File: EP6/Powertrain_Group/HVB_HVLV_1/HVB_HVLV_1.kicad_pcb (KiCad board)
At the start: 2 copper layers, 132 x 62 mm, 20 parts, among them J1 HV+, J2 HV-, J3 from LV, J5 DCDC-, J6 DCDC+, K1 G7L-2A-X DC24, K2 DBT72410, Q1 IXTH6N100D2, U1 PC817

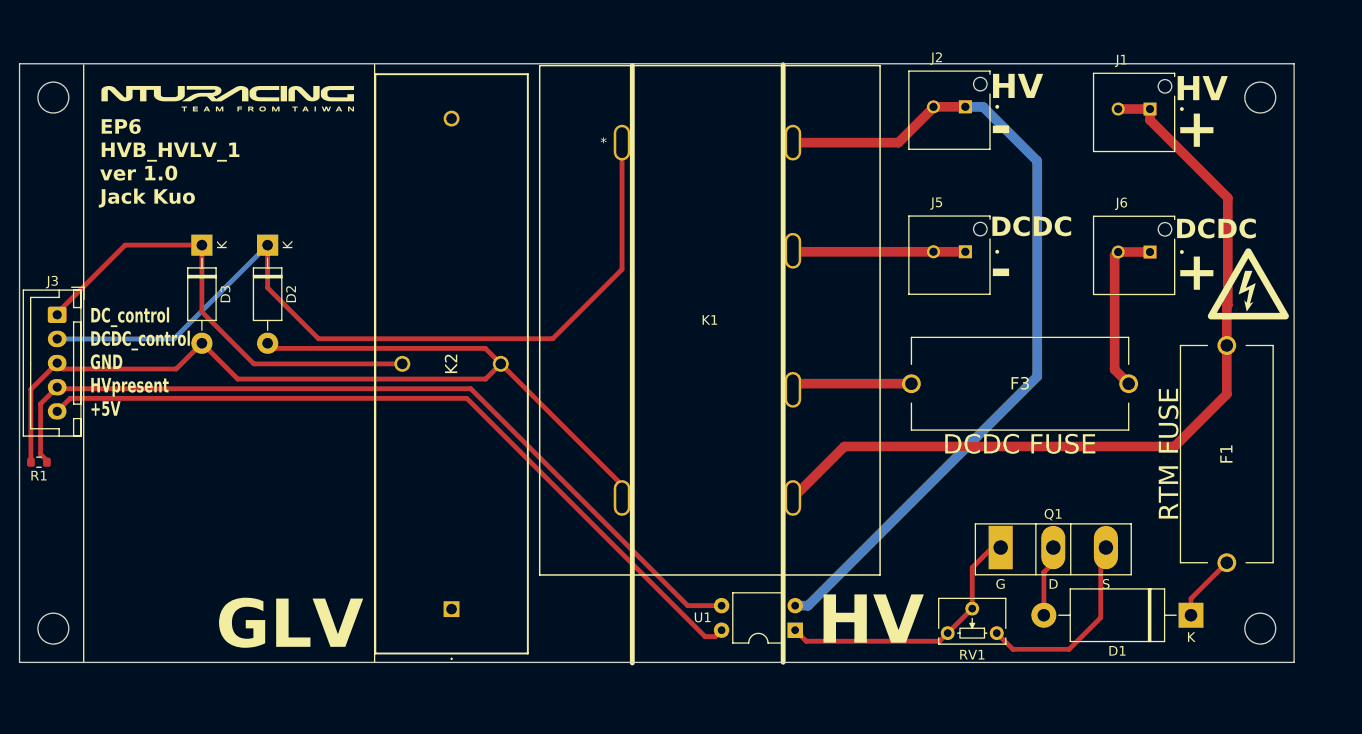
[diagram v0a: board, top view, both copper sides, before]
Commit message: update HVB_HVLV_1 V2.1
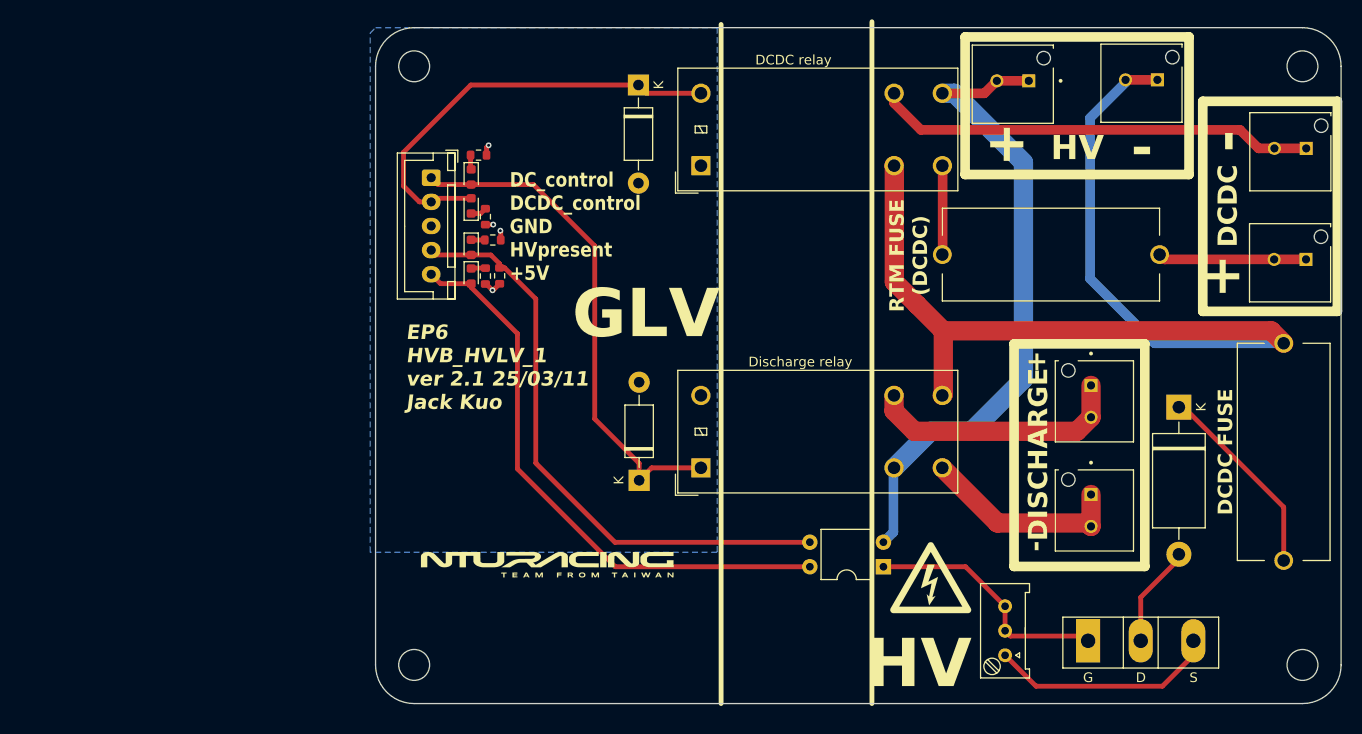
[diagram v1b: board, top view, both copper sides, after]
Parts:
- added D4: RED LED, LED_SMD:LED_0603_1608Metric, F.Cu at (109.9, 47.8)
- added D5: RED LED, LED_SMD:LED_0603_1608Metric, F.Cu at (109.9, 50.7)
- added D6: RED LED, LED_SMD:LED_0603_1608Metric, F.Cu at (109.9, 43.5)
- added D7: RED LED, LED_SMD:LED_0603_1608Metric, F.Cu at (109.9, 40.5)
- added J4: PrechargeRes-, nturt_kicad_lib_EP6:HRS_DF33C-2P-3.3DSA, F.Cu at (174.1, 75.0)
- added J7: PrechargeRes+, nturt_kicad_lib_EP6:HRS_DF33C-2P-3.3DSA, F.Cu at (174.1, 63.7)
- added R2: 10k, Resistor_SMD:R_0603_1608Metric, F.Cu at (112.1, 47.0)
- added R3: 10k, Resistor_SMD:R_0603_1608Metric, F.Cu at (111.4, 50.7)
- added R4: 10k, Resistor_SMD:R_0603_1608Metric, F.Cu at (111.4, 44.6)
- added R5: 10k, Resistor_SMD:R_0603_1608Metric, F.Cu at (110.7, 38.2)
- K1: value G7L-2A-X DC24 -> G2RG-2A-X DC24; footprint nturt_kicad_lib_EP6:RELAY_G7L-2A-X_OMR -> Relay_THT:Relay_DPST_Omron_G2RL-2A
- K2: value DBT72410 -> G2RG-2A-X DC24; footprint SamacSys_Parts_EP6:DBT72410 -> Relay_THT:Relay_DPST_Omron_G2RL-2A
- RV1: value 10k -> 10K; footprint PCM_Potentiometer_THT_AKL:Potentiometer_Bourns_3266W_Vertical -> nturt_kicad_lib_EP6:Throughhole Potentiometer 3296W
- moved R1 51.5 mm to (112.9, 50.7), turned to -90 degrees
- moved D3 51.4 mm to (127.3, 71.9), turned to 90 degrees
- moved D2 41.8 mm to (127.2, 30.9)
- moved J3 41.3 mm to (105.8, 40.5)
- moved H3 37.6 mm to (104.0, 91.0)
- moved H2 37.5 mm to (104.0, 29.0)
- moved J5 36.9 mm to (194.7, 37.5)
- moved K2 29.7 mm to (133.7, 70.6)
- moved D1 21.6 mm to (183.2, 64.3), turned to -90 degrees
- moved J6 16.2 mm to (194.7, 49.0)
- moved F3 13.8 mm to (170.0, 48.5)
- moved Q1 13.2 mm to (173.8, 88.5)
- moved U1 11.3 mm to (152.6, 80.8)
- moved K1 8.52 mm to (133.7, 39.3), turned to 90 degrees
- moved J2 7.09 mm to (166.0, 30.5)
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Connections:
- RV1 pad 1: Net-(Q1-G) -> Net-(Q1-S)
- RV1 pad 3: Net-(Q1-S) -> Net-(Q1-G)
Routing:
- net GND: track 105.0 -> 4.92 mm, vias 0 -> 4
- net /DCDC_CONTROL: track 85.2 -> 45.4 mm
- net Net-(J5-Pin_1): track 17.9 -> 45.6 mm
- net Net-(J7-Pin_1): track 0.00 -> 26.8 mm
- net /HVpresent: track 86.9 -> 62.0 mm
- net /HV+: track 85.6 -> 110.0 mm
- net Net-(J4-Pin_1): track 0.00 -> 21.2 mm
- net +5V: track 79.9 -> 60.2 mm
- net /HV-: track 86.4 -> 68.7 mm
- net Net-(D1-K): track 6.97 -> 20.7 mm
- net /DC_CONTROL: track 48.0 -> 53.0 mm
- net Net-(Q1-S): track 20.3 -> 23.7 mm
- net Net-(F3-Pad2): track 12.5 -> 9.23 mm
- net Net-(D1-A): track 7.53 -> 10.6 mm
- net Net-(Q1-G): track 28.3 -> 25.9 mm
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- added copper zone on B.Cu, net GND
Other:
- board size 132 x 62 mm -> 100 x 70 mm
- board text added: "DCDC relay"
- board text added: "DISCHARGE"
- board text added: "Discharge relay"
- board text added: "EP6 HVB_HVLV_1 ver 2.1 25/03/11 Jack Kuo"
- board text added: "RTM FUSE (DCDC)"
- board text removed: "EP6 HVB_HVLV_1 ver 1.0 Jack Kuo"
- board text removed: "RTM FUSE"
